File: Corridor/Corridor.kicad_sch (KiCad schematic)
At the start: 31 parts, among them IC2 SHT31-DIS-B2.5KS, J1 WJ127-5.0-2P, J3 Servo2, J4 RFID, J6 Scale, J7 IR_LEDs, J8 Corridor1, J9 Servo1, Q1 IRLML2502PBF, U1 ADS1114IDGS, U2 AP2210N-3.3TRG1, U3 AD8293G80ARJZ-R7, U4 PCA9685PW, U5 PCA9306

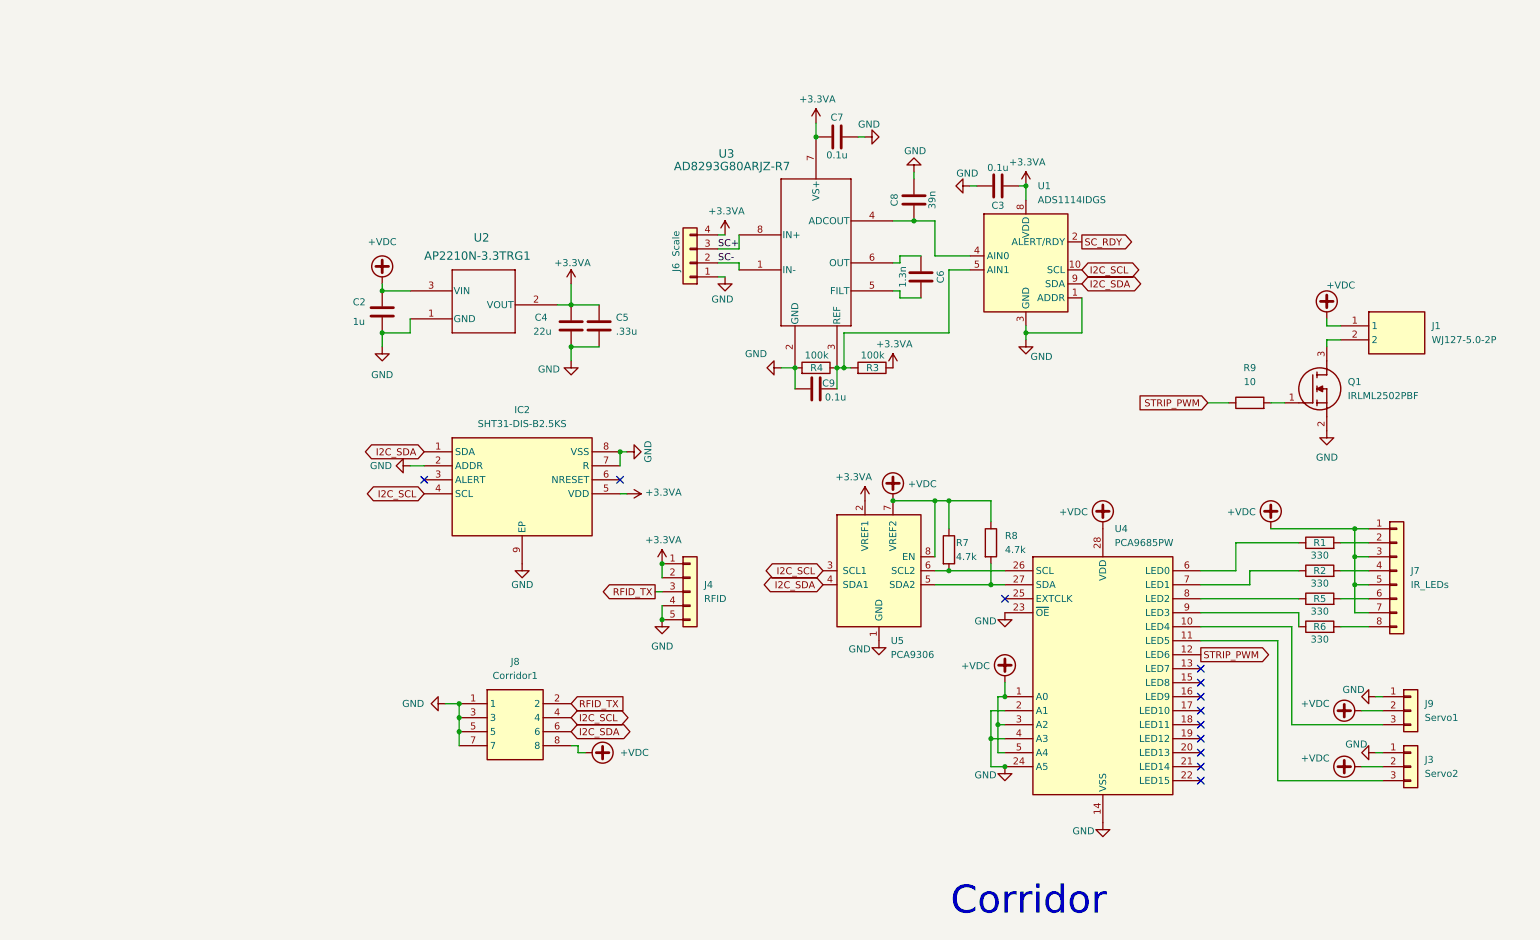
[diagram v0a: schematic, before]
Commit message: v1.0
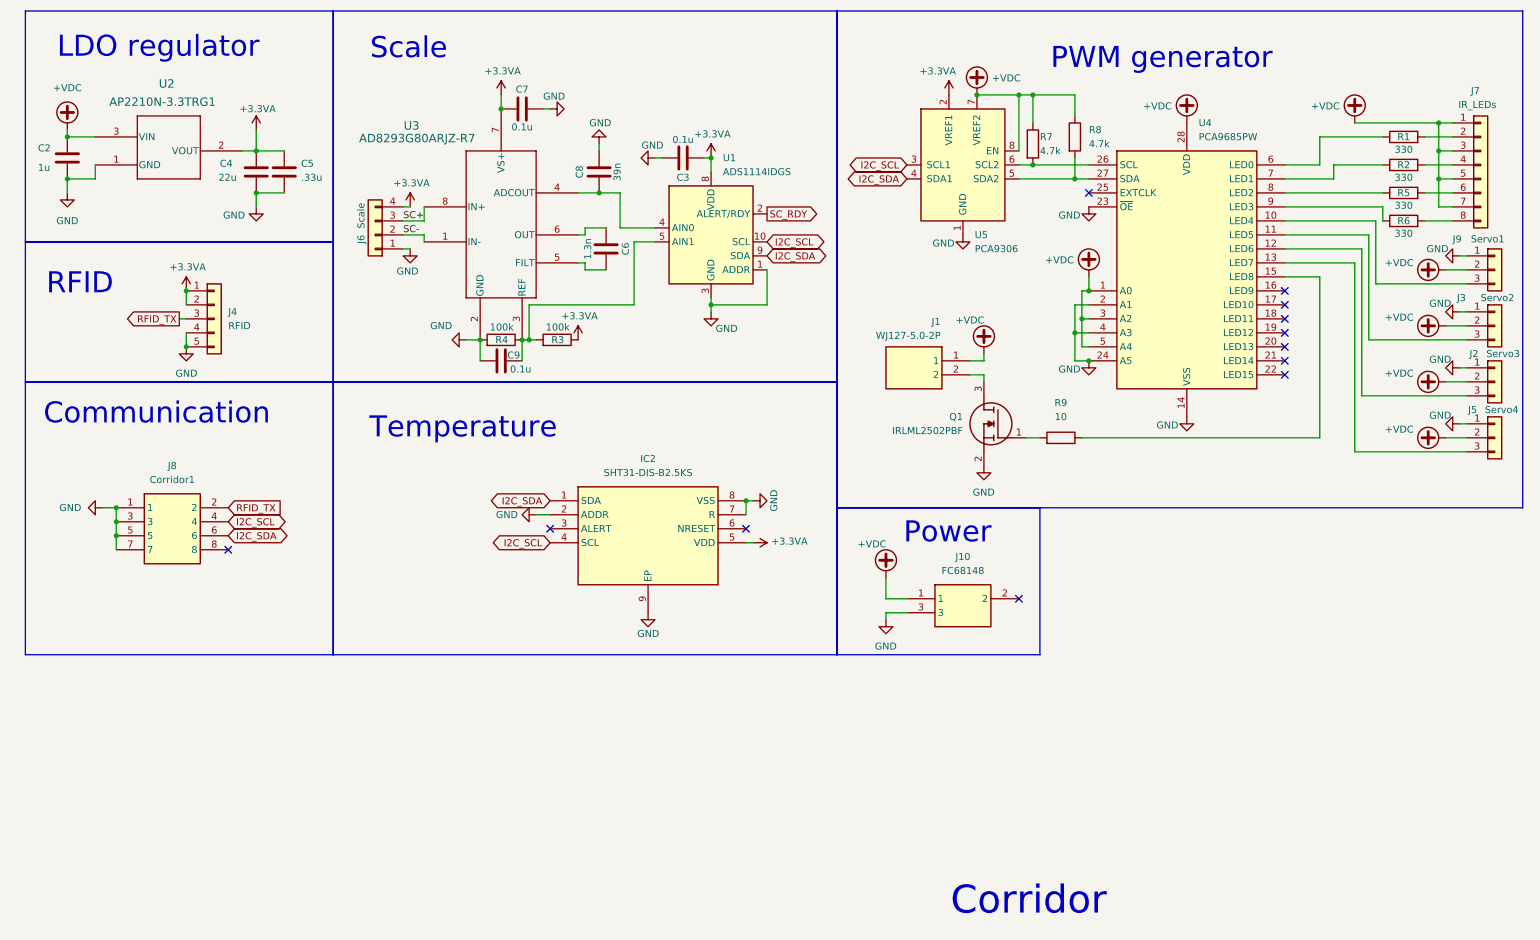
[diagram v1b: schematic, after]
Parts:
- added J10: FC68148, FC68148:FC68148, symbol FC68148:FC68148
- added J2: Servo3, Connector_PinHeader_2.54mm:PinHeader_1x03_P2.54mm_Vertical, symbol Connector_Generic:Conn_01x03
- added J5: Servo4, Connector_PinHeader_2.54mm:PinHeader_1x03_P2.54mm_Vertical, symbol Connector_Generic:Conn_01x03
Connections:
- net +VDC: now also J10.1, J2.2 (Pin_2), J5.2 (Pin_2); no longer J8.8
- net GND: now also J10.3, J2.1 (Pin_1), J5.1 (Pin_1)
- net at U4.13 (LED7): now also J5.3 (Pin_3)
- net at U4.15 (LED8): now also R9.1
- net STRIP_PWM: no longer names the net of U4.12 (LED6)
- net STRIP_PWM: now also J2.3 (Pin_3); no longer R9.1
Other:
- note added: "Communication"
- note added: "LDO regulator"
- note added: "PWM generator"
- note added: "Power"
- note added: "RFID"
- note added: "Scale"
- note added: "Temperature"
- moved on the sheet: C2, C3, C4, C5, C6, C7, C8, C9, IC2, J1, J3, J4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
